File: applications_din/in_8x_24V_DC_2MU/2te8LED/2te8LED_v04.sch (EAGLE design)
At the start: 19 parts, among them IC1 74HC595D

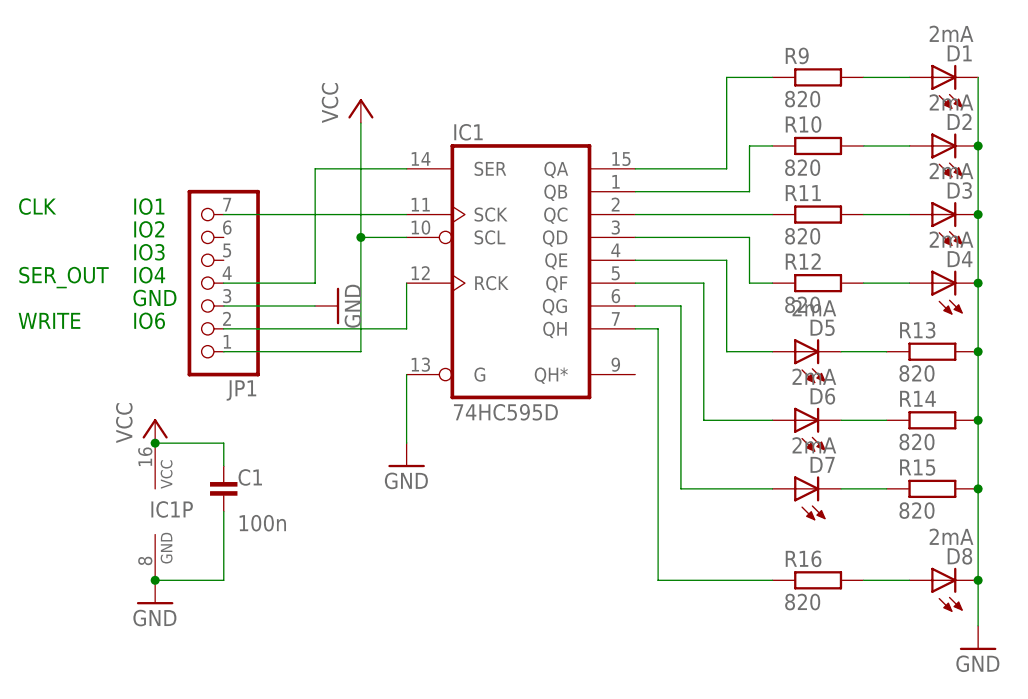
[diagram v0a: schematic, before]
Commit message: 3D models added
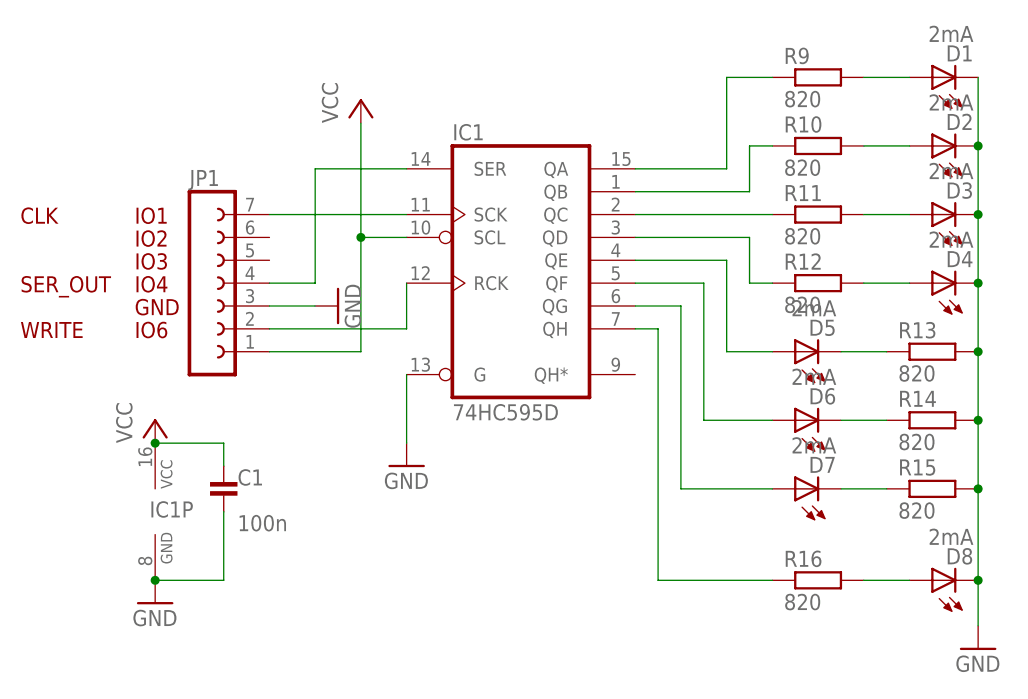
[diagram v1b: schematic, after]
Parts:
- JP1: device pinhead:PINHD-1X7_2.54 -> con-lsta:FE07-1
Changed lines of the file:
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@@
 <drawing>
 <settings>
-<setting alwaysvectorfont="yes"/>
+<setting alwaysvectorfont="no"/>
 <setting keepoldvectorfont="yes"/>
 <setting verticaltext="up"/>
@@
 <part name="D7" library="led" deviceset="LED" device="3MM" value="2mA"/>
 <part name="D8" library="led" deviceset="LED" device="3MM" value="2mA"/>
-<part name="IC1" library="74xx-eu" deviceset="74*595" device="D" technology="HC"/>
+<part name="IC1" library="74xx-eu" library_urn="urn:adsk.eagle:library:85" deviceset="74*595" device="D" package3d_urn="urn:adsk.eagle:package:2010/1" override_package3d_urn="urn:adsk.eagle:package:48524435/2" override_package_urn="urn:adsk.eagle:footprint:1637/1" technology="HC"/>
 <part name="GND3" library="supply1" deviceset="GND" device=""/>
 <part name="R9" library="MyRCL" deviceset="R-EU_" device="R0805" package3d_urn="urn:adsk.eagle:package:18594703/1" value="820"/>
@@
 <part name="P+3" library="supply1" deviceset="VCC" device=""/>
 <part name="C1" library="MyRCL" deviceset="C-EU" device="C0805" package3d_urn="urn:adsk.eagle:package:23617/2" value="100n"/>
-<part name="JP1" library="pinhead" deviceset="PINHD-1X7" device="_2.54"/>
+<part name="JP1" library="con-lsta" library_urn="urn:adsk.eagle:library:161" deviceset="FE07-1" device="" package3d_urn="urn:adsk.eagle:package:8223/1" override_package3d_urn="urn:adsk.eagle:package:48524428/2" override_package_urn="urn:adsk.eagle:footprint:8137/1"/>
 </parts>
 <sheets>
 <sheet>
 <plain>
-<text x="25.4" y="58.42" size="1.778" layer="91">IO1</text>
-<text x="25.4" y="55.88" size="1.778" layer="91">IO2</text>
-<text x="25.4" y="53.34" size="1.778" layer="91">IO3</text>
-<text x="25.4" y="50.8" size="1.778" layer="91">IO4</text>
-<text x="25.4" y="45.72" size="1.778" layer="91">IO6</text>
-<text x="25.4" y="48.26" size="1.778" layer="91">GND</text>
-<text x="12.7" y="58.42" size="1.778" layer="91">CLK</text>
-<text x="12.7" y="50.8" size="1.778" layer="91">SER_OUT</text>
-<text x="12.7" y="45.72" size="1.778" layer="91">WRITE</text>
+<text x="25.654" y="57.404" size="1.778" layer="94">IO1</text>
+<text x="25.654" y="54.864" size="1.778" layer="94">IO2</text>
+<text x="25.654" y="52.324" size="1.778" layer="94">IO3</text>
+<text x="25.654" y="49.784" size="1.778" layer="94">IO4</text>
+<text x="25.654" y="44.704" size="1.778" layer="94">IO6</text>
+<text x="25.654" y="47.244" size="1.778" layer="94">GND</text>
+<text x="12.954" y="57.404" size="1.778" layer="94">CLK</text>
+<text x="12.954" y="49.784" size="1.778" layer="94">SER_OUT</text>
+<text x="12.954" y="44.704" size="1.778" layer="94">WRITE</text>
 </plain>
 <instances>
@@
 <attribute name="VALUE" x="37.084" y="23.241" size="1.778" layer="96"/>
 </instance>
-<instance part="JP1" gate="A" x="33.02" y="50.8" smashed="yes" rot="R180">
-<attribute name="NAME" x="39.37" y="40.005" size="1.778" layer="95" rot="R180"/>
-<attribute name="VALUE" x="39.37" y="63.5" size="1.778" layer="96" rot="R180"/>
+<instance part="JP1" gate="G$1" x="33.02" y="50.8" smashed="yes">
+<attribute name="NAME" x="31.75" y="61.595" size="1.778" layer="95"/>
+<attribute name="VALUE" x="26.67" y="38.1" size="1.778" layer="96"/>
 </instance>
 </instances>
@@
 </segment>
 <segment>
-<wire x1="45.72" y1="48.26" x2="35.56" y2="48.26" width="0.1524" layer="91"/>
+<wire x1="45.72" y1="48.26" x2="40.64" y2="48.26" width="0.1524" layer="91"/>
 <pinref part="GND3" gate="1" pin="GND"/>
-<pinref part="JP1" gate="A" pin="3"/>
+<pinref part="JP1" gate="G$1" pin="3"/>
 </segment>
 <segment>
@@
 <net name="IO1" class="0">
 <segment>
-<wire x1="35.56" y1="58.42" x2="55.88" y2="58.42" width="0.1524" layer="91"/>
+<wire x1="40.64" y1="58.42" x2="55.88" y2="58.42" width="0.1524" layer="91"/>
 <pinref part="IC1" gate="A" pin="SCK"/>
-<pinref part="JP1" gate="A" pin="7"/>
+<pinref part="JP1" gate="G$1" pin="7"/>
 </segment>
 </net>
@@
 <wire x1="50.8" y1="55.88" x2="50.8" y2="43.18" width="0.1524" layer="91"/>
 <junction x="50.8" y="55.88"/>
-<pinref part="JP1" gate="A" pin="1"/>
-<wire x1="50.8" y1="43.18" x2="35.56" y2="43.18" width="0.1524" layer="91"/>
+<pinref part="JP1" gate="G$1" pin="1"/>
+<wire x1="50.8" y1="43.18" x2="40.64" y2="43.18" width="0.1524" layer="91"/>
 </segment>
 <segment>
@@
 <wire x1="55.88" y1="63.5" x2="45.72" y2="63.5" width="0.1524" layer="91"/>
 <wire x1="45.72" y1="63.5" x2="45.72" y2="50.8" width="0.1524" layer="91"/>
-<wire x1="45.72" y1="50.8" x2="35.56" y2="50.8" width="0.1524" layer="91"/>
+<wire x1="45.72" y1="50.8" x2="40.64" y2="50.8" width="0.1524" layer="91"/>
 <pinref part="IC1" gate="A" pin="SER"/>
-<pinref part="JP1" gate="A" pin="4"/>
+<pinref part="JP1" gate="G$1" pin="4"/>
 </segment>
 </net>
 <net name="IO6" class="0">
 <segment>
-<wire x1="35.56" y1="45.72" x2="55.88" y2="45.72" width="0.1524" layer="91"/>
+<wire x1="40.64" y1="45.72" x2="55.88" y2="45.72" width="0.1524" layer="91"/>
 <wire x1="55.88" y1="45.72" x2="55.88" y2="50.8" width="0.1524" layer="91"/>
 <pinref part="IC1" gate="A" pin="RCK"/>
-<pinref part="JP1" gate="A" pin="2"/>
+<pinref part="JP1" gate="G$1" pin="2"/>
 </segment>
 </net>
@@
 </drawing>
 <compatibility>
+<note version="8.2" severity="warning">
+Since Version 8.2, EAGLE supports online libraries. The ids
+of those online libraries will not be understood (or retained)
+with this version.
+</note>
 <note version="8.3" severity="warning">
 Since Version 8.3, EAGLE supports URNs for individual library
@@
 packages will not be understood (or retained) with this version.
 </note>
+<note version="9.4" severity="warning">
+Since Version 9.4, EAGLE supports the overriding of 3D packages
+in schematics and board files. Those overridden 3d packages
+will not be understood (or retained) with this version.
+</note>
 <note version="8.4" severity="warning">
